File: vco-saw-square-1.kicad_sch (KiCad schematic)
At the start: 41 parts, among them J1 CVpitch, J13 wave-select, J2 FM in, J3 PWM in, J5 VCO-out, Q1 BC807, Q2 BC817, U1 HEF4093B, U2 TL074

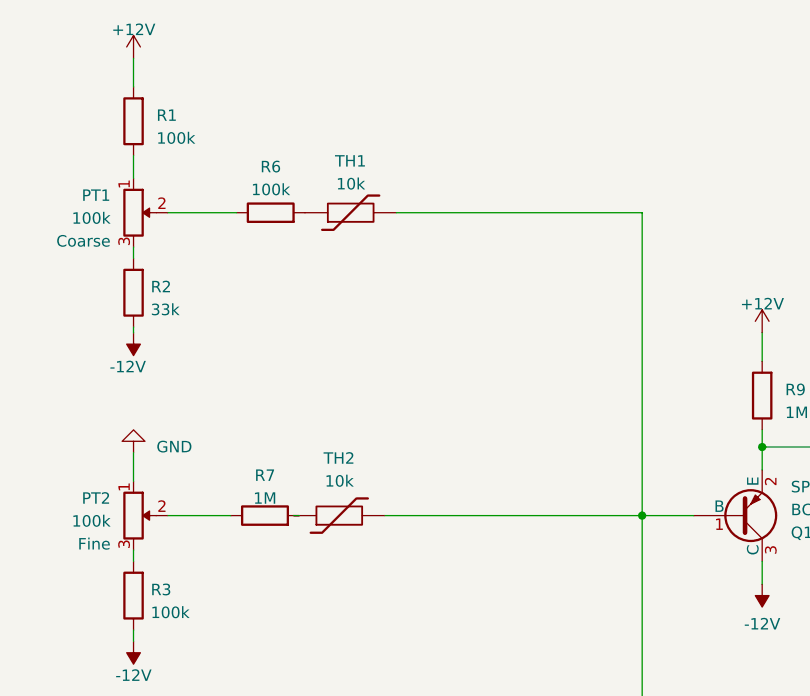
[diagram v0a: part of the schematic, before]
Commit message: dfgdrfghdf
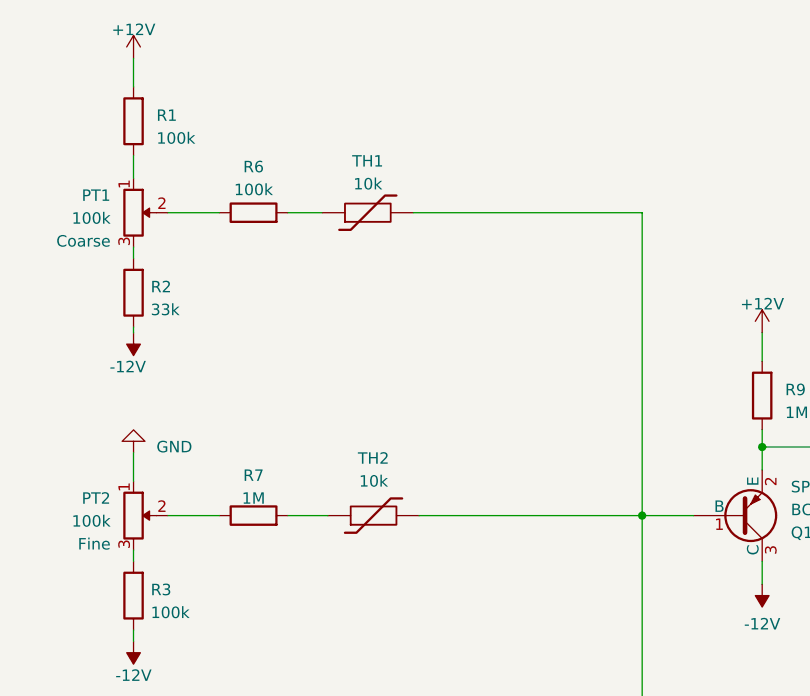
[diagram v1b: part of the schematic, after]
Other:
- moved on the sheet: R6, R7, TH1, TH2
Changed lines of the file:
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@@
     (stroke (width 0) (type default))
   )
-  (wire (pts (xy 46.355 74.295) (xy 45.72 74.295))
+  (wire (pts (xy 45.085 74.295) (xy 49.53 74.295))
     (stroke (width 0) (type default))
   )
@@
     (stroke (width 0) (type default))
   )
-  (wire (pts (xy 31.75 40.64) (xy 39.37 40.64))
+  (wire (pts (xy 31.75 40.64) (xy 37.465 40.64))
     (stroke (width 0) (type default))
   )
@@
     (stroke (width 0) (type default))
   )
-  (wire (pts (xy 55.88 74.295) (xy 84.455 74.295))
+  (wire (pts (xy 59.69 74.295) (xy 84.455 74.295))
     (stroke (width 0) (type default))
   )
@@
     (stroke (width 0) (type default))
   )
-  (wire (pts (xy 84.455 40.64) (xy 57.15 40.64))
+  (wire (pts (xy 84.455 40.64) (xy 59.055 40.64))
     (stroke (width 0) (type default))
   )
@@
     (stroke (width 0) (type default))
   )
+  (wire (pts (xy 45.085 40.64) (xy 48.895 40.64))
+    (stroke (width 0) (type default))
+  )
   (wire (pts (xy 138.43 55.88) (xy 138.43 58.42))
     (stroke (width 0) (type default))
@@
     (stroke (width 0) (type default))
   )
-  (wire (pts (xy 31.75 74.295) (xy 38.735 74.295))
+  (wire (pts (xy 31.75 74.295) (xy 37.465 74.295))
     (stroke (width 0) (type default))
   )
@@
     )
   )
-  (symbol (lib_id "000-thermistor-immo:NTC-thermistor-10k-0805") (at 50.8 74.295 90) (unit 1)
-    (in_bom yes) (on_board yes) (dnp no) (fields_autoplaced)
-    (property "Reference" "TH2" (at 50.8 67.945 90)
-      (effects (font (size 1.27 1.27)))
-    )
-    (property "Value" "10k" (at 50.8 70.485 90)
-      (effects (font (size 1.27 1.27)))
-    )
-    (property "Footprint" "000_Resistors_Immo:Resistor_0805_2012_handsolder" (at 50.8 74.295 0)
-      (effects (font (size 1.27 1.27)) hide)
-    )
-    (property "Datasheet" "~" (at 50.8 74.295 0)
-      (effects (font (size 1.27 1.27)) hide)
-    )
-    (property "RSpart" "202-5368" (at 50.8 74.295 0)
-      (effects (font (size 1.27 1.27)) hide)
-    )
-    (property "supplier" "https://uk.rs-online.com/web/p/thermistor-ics/2025368?gb=s" (at 50.8 74.295 0)
-      (effects (font (size 1.27 1.27)) hide)
-    )
-    (property "cost" "£0.149" (at 50.8 74.295 0)
+  (symbol (lib_id "000-thermistor-immo:NTC-thermistor-10k-0805") (at 54.61 74.295 90) (unit 1)
+    (in_bom yes) (on_board yes) (dnp no) (fields_autoplaced)
+    (property "Reference" "TH2" (at 54.61 67.945 90)
+      (effects (font (size 1.27 1.27)))
+    )
+    (property "Value" "10k" (at 54.61 70.485 90)
+      (effects (font (size 1.27 1.27)))
+    )
+    (property "Footprint" "000_Resistors_Immo:Resistor_0805_2012_handsolder" (at 54.61 74.295 0)
+      (effects (font (size 1.27 1.27)) hide)
+    )
+    (property "Datasheet" "~" (at 54.61 74.295 0)
+      (effects (font (size 1.27 1.27)) hide)
+    )
+    (property "RSpart" "202-5368" (at 54.61 74.295 0)
+      (effects (font (size 1.27 1.27)) hide)
+    )
+    (property "supplier" "https://uk.rs-online.com/web/p/thermistor-ics/2025368?gb=s" (at 54.61 74.295 0)
+      (effects (font (size 1.27 1.27)) hide)
+    )
+    (property "cost" "£0.149" (at 54.61 74.295 0)
       (effects (font (size 1.27 1.27)) hide)
     )
@@
     )
   )
-  (symbol (lib_id "000_Resistors_Immo:100k") (at 43.18 40.64 0) (unit 1)
-    (in_bom yes) (on_board yes) (dnp no) (fields_autoplaced)
-    (property "Reference" "R6" (at 43.18 35.56 0)
-      (effects (font (size 1.27 1.27)))
-    )
-    (property "Value" "100k" (at 43.18 38.1 0)
-      (effects (font (size 1.27 1.27)))
-    )
-    (property "Footprint" "Resistor_SMD:R_0805_2012Metric_Pad1.20x1.40mm_HandSolder" (at 43.18 42.418 0)
-      (effects (font (size 1.27 1.27)) hide)
-    )
-    (property "Datasheet" "~" (at 43.18 40.64 90)
-      (effects (font (size 1.27 1.27)) hide)
-    )
-    (property "JLCpart" "C280020" (at 44.45 43.18 0)
-      (effects (font (size 1.27 1.27)) hide)
-    )
-    (property "Cost" "0.0027" (at 43.18 43.18 0)
+  (symbol (lib_id "000_Resistors_Immo:100k") (at 41.275 40.64 0) (unit 1)
+    (in_bom yes) (on_board yes) (dnp no) (fields_autoplaced)
+    (property "Reference" "R6" (at 41.275 35.56 0)
+      (effects (font (size 1.27 1.27)))
+    )
+    (property "Value" "100k" (at 41.275 38.1 0)
+      (effects (font (size 1.27 1.27)))
+    )
+    (property "Footprint" "Resistor_SMD:R_0805_2012Metric_Pad1.20x1.40mm_HandSolder" (at 41.275 42.418 0)
+      (effects (font (size 1.27 1.27)) hide)
+    )
+    (property "Datasheet" "~" (at 41.275 40.64 90)
+      (effects (font (size 1.27 1.27)) hide)
+    )
+    (property "JLCpart" "C280020" (at 42.545 43.18 0)
+      (effects (font (size 1.27 1.27)) hide)
+    )
+    (property "Cost" "0.0027" (at 41.275 43.18 0)
       (effects (font (size 1.27 1.27)) hide)
     )
@@
     )
   )
-  (symbol (lib_id "000-thermistor-immo:NTC-thermistor-10k-0805") (at 52.07 40.64 90) (unit 1)
-    (in_bom yes) (on_board yes) (dnp no) (fields_autoplaced)
-    (property "Reference" "TH1" (at 52.07 34.925 90)
-      (effects (font (size 1.27 1.27)))
-    )
-    (property "Value" "10k" (at 52.07 37.465 90)
-      (effects (font (size 1.27 1.27)))
-    )
-    (property "Footprint" "000_Resistors_Immo:Resistor_0805_2012_handsolder" (at 52.07 40.64 0)
-      (effects (font (size 1.27 1.27)) hide)
-    )
-    (property "Datasheet" "~" (at 52.07 40.64 0)
-      (effects (font (size 1.27 1.27)) hide)
-    )
-    (property "RSpart" "202-5368" (at 52.07 40.64 0)
-      (effects (font (size 1.27 1.27)) hide)
-    )
-    (property "supplier" "https://uk.rs-online.com/web/p/thermistor-ics/2025368?gb=s" (at 52.07 40.64 0)
-      (effects (font (size 1.27 1.27)) hide)
-    )
-    (property "cost" "£0.149" (at 52.07 40.64 0)
+  (symbol (lib_id "000-thermistor-immo:NTC-thermistor-10k-0805") (at 53.975 40.64 90) (unit 1)
+    (in_bom yes) (on_board yes) (dnp no) (fields_autoplaced)
+    (property "Reference" "TH1" (at 53.975 34.925 90)
+      (effects (font (size 1.27 1.27)))
+    )
+    (property "Value" "10k" (at 53.975 37.465 90)
+      (effects (font (size 1.27 1.27)))
+    )
+    (property "Footprint" "000_Resistors_Immo:Resistor_0805_2012_handsolder" (at 53.975 40.64 0)
+      (effects (font (size 1.27 1.27)) hide)
+    )
+    (property "Datasheet" "~" (at 53.975 40.64 0)
+      (effects (font (size 1.27 1.27)) hide)
+    )
+    (property "RSpart" "202-5368" (at 53.975 40.64 0)
+      (effects (font (size 1.27 1.27)) hide)
+    )
+    (property "supplier" "https://uk.rs-online.com/web/p/thermistor-ics/2025368?gb=s" (at 53.975 40.64 0)
+      (effects (font (size 1.27 1.27)) hide)
+    )
+    (property "cost" "£0.149" (at 53.975 40.64 0)
       (effects (font (size 1.27 1.27)) hide)
     )
@@
     )
   )
-  (symbol (lib_id "000_Resistors_Immo:Resistor_0805") (at 42.545 74.295 0) (unit 1)
-    (in_bom yes) (on_board yes) (dnp no) (fields_autoplaced)
-    (property "Reference" "R7" (at 42.545 69.85 0)
-      (effects (font (size 1.27 1.27)))
-    )
-    (property "Value" "1M" (at 42.545 72.39 0)
-      (effects (font (size 1.27 1.27)))
-    )
-    (property "Footprint" "Resistor_SMD:R_0805_2012Metric_Pad1.20x1.40mm_HandSolder" (at 42.545 76.073 0)
-      (effects (font (size 1.27 1.27)) hide)
-    )
-    (property "Datasheet" "~" (at 42.545 74.295 90)
-      (effects (font (size 1.27 1.27)) hide)
-    )
+  (symbol (lib_id "000_Resistors_Immo:Resistor_0805") (at 41.275 74.295 0) (unit 1)
+    (in_bom yes) (on_board yes) (dnp no) (fields_autoplaced)
+    (property "Reference" "R7" (at 41.275 69.85 0)
+      (effects (font (size 1.27 1.27)))
+    )
+    (property "Value" "1M" (at 41.275 72.39 0)
+      (effects (font (size 1.27 1.27)))
+    )
+    (property "Footprint" "Resistor_SMD:R_0805_2012Metric_Pad1.20x1.40mm_HandSolder" (at 41.275 76.073 0)
+      (effects (font (size 1.27 1.27)) hide)
+    )
+    (property "Datasheet" "~" (at 41.275 74.295 90)
+      (effects (font (size 1.27 1.27)) hide)
+    )
